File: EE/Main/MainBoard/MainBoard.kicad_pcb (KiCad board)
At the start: 2 copper layers, 135.8 x 87.5 mm, 59 parts, among them J1 Conn_01x04_Male, J2 Conn_01x04_Male, J3 Conn_01x04_Male, J4 Conn_01x04_Male, J5 Conn_01x04_Male, J6 Conn_01x04_Male, J7 TAG_CONNECT, J8 Conn_01x02_Male, P1 USB_C_Plug_USB2.0, Q1 2N7002NXAKR, Q2 2N7002NXAKR, Q3 2N7002NXAKR, Q4 2N7002NXAKR, SW1 EG1206A, U1 STM32C011F4U6TR, U2 DA04-11EWA, U3 DA04-11GWA, U4 MCP73832-2-OT, U5 TPS62172DSG

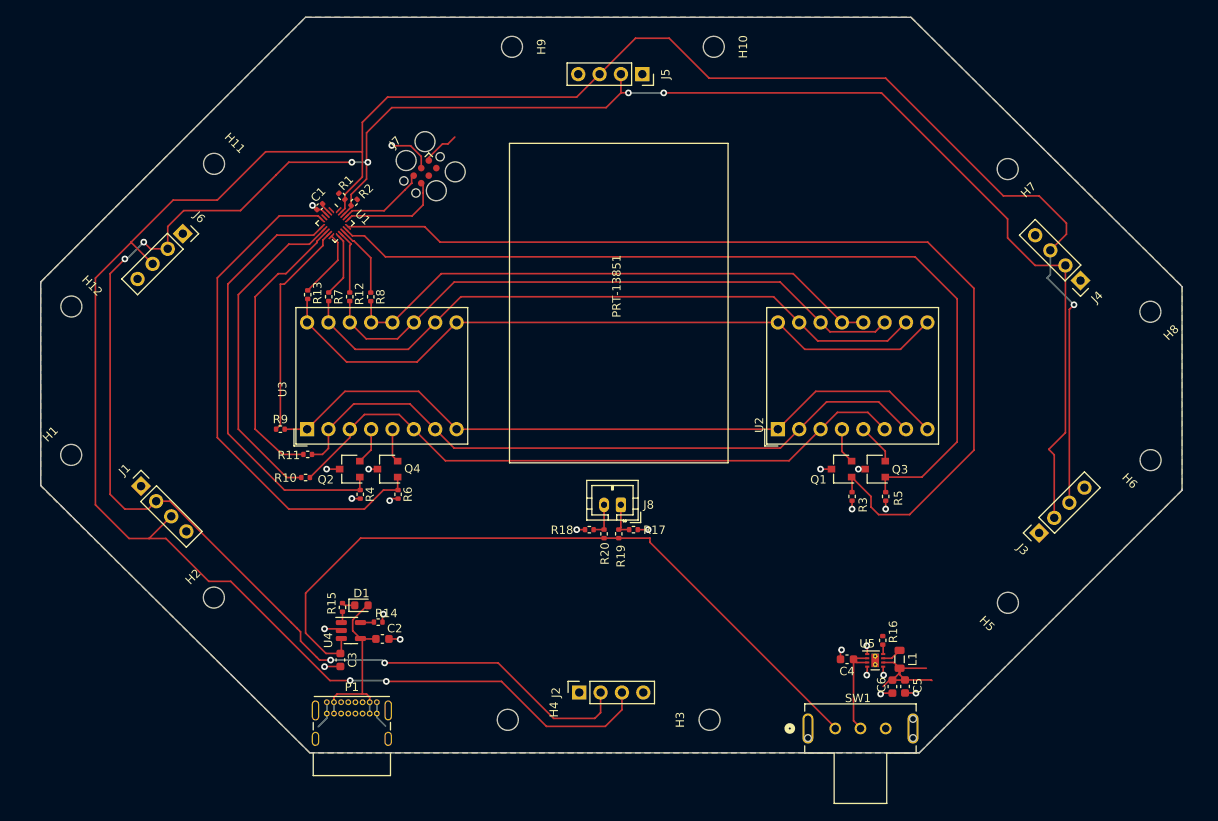
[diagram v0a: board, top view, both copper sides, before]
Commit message: Routine Update
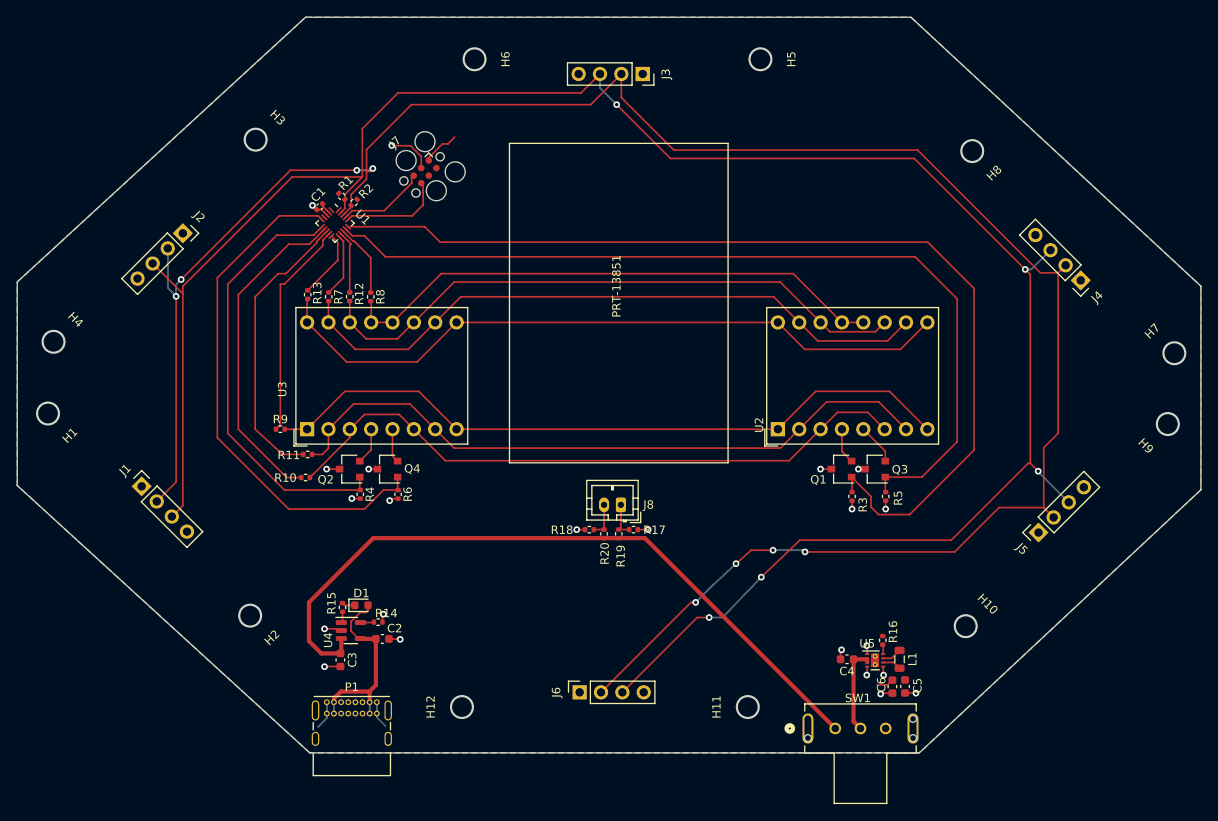
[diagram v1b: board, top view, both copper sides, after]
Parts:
- added ?: , , F.Cu at (159.6, 133.3)
- added ?: , , F.Cu at (186.3, 67.2)
- added ?: , , F.Cu at (77.0, 89.9)
- added ?: , , F.Cu at (76.4, 98.4)
- added ?: , , F.Cu at (100.4, 122.5)
- added ?: , , F.Cu at (210.3, 91.2)
- added ?: , , F.Cu at (127.1, 56.3)
- added ?: , , F.Cu at (185.5, 123.7)
- added ?: , , F.Cu at (161.1, 56.3)
- added ?: , , F.Cu at (125.6, 133.3)
- added ?: , , F.Cu at (209.6, 99.7)
- added ?: , , F.Cu at (101.1, 65.8)
- H1, H10, H11, H12, H2, H3, H4, H5, H6, H7, H8, H9: footprint MountingHole:MountingHole_2.5mm -> MountingHole:MountingHole_2.7mm
- moved H6 93.5 mm to (127.1, 56.3), turned to -90 degrees
- moved H11 90.6 mm to (159.6, 133.3), turned to 90 degrees
- moved H9 90.0 mm to (209.6, 99.7), turned to 135 degrees
- moved H3 87.6 mm to (101.1, 65.8), turned to -45 degrees
- moved H10 75.1 mm to (185.5, 123.7), turned to -45 degrees
- moved J2 72.2 mm to (92.4, 77.0), turned to -45 degrees
- moved J6 72.1 mm to (139.6, 131.6), turned to 90 degrees
- moved J3 72.1 mm to (147.1, 58.0), turned to -90 degrees
- moved J5 72.1 mm to (194.2, 112.6), turned to 135 degrees
- moved H5 71.0 mm to (161.1, 56.3), turned to -90 degrees
- moved H4 70.3 mm to (77.0, 89.9), turned to -45 degrees
- moved H12 66.5 mm to (125.6, 133.3), turned to 90 degrees
- moved H7 29.5 mm to (210.3, 91.2), turned to 45 degrees
- moved H8 28.5 mm to (186.3, 67.2)
- moved H1 5.64 mm to (76.4, 98.4), turned to -135 degrees
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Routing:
- net /SDA: track 293.3 -> 256.6 mm, vias 3 -> 5
- net /SCL: track 277.4 -> 262.6 mm
- net VCC: track 20.8 -> 10.4 mm
- net VBUS: track 22.2 -> 24.2 mm
- net /Power/V_PRE_REG: track 11.9 -> 10.7 mm
- net /Power/VBAT: track 87.1 -> 85.9 mm
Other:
- board size 135.8 x 87.5 mm -> 140.8 x 87.5 mm

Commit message: Random Check in
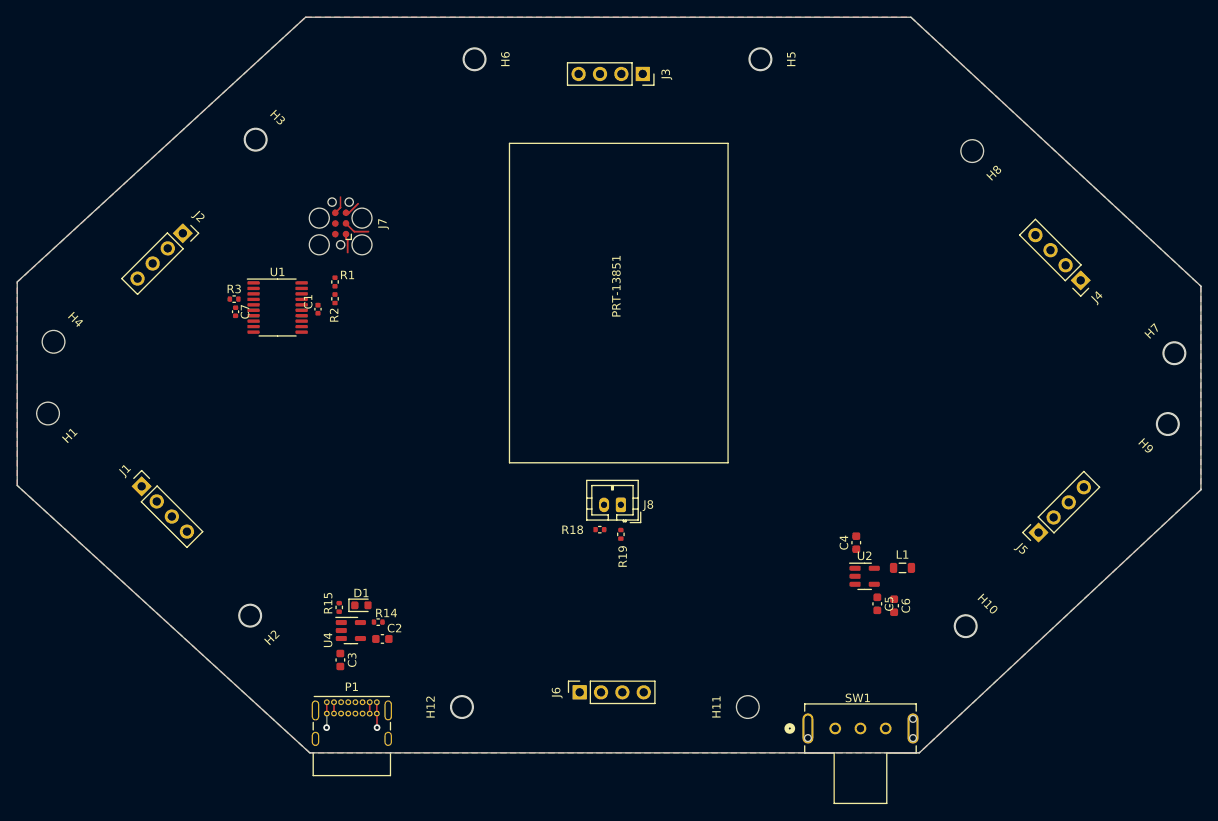
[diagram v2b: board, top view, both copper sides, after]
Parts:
- removed the ? at (159.6, 133.3)
- removed the ? at (186.3, 67.2)
- removed the ? at (77.0, 89.9)
- removed the ? at (76.4, 98.4)
- removed Q1, Q2, Q3, Q4: 2N7002NXAKR, Package_TO_SOT_SMD:SC-59
- removed R10, R11, R12, R13, R7, R8, R9: 560, Resistor_SMD:R_0402_1005Metric
- removed R16: 100k, Resistor_SMD:R_0402_1005Metric
- removed R17, R20: 0, Resistor_SMD:R_0402_1005Metric
- removed R4, R5, R6: 10k, Resistor_SMD:R_0402_1005Metric
- removed U3: DA04-11GWA, Display_7Segment:DA04-11CGKWA
- removed U5: TPS62172DSG, Package_SON:WSON-8-1EP_2x2mm_P0.5mm_EP0.9x1.6mm_ThermalVias
- added C7: 0.1u, Capacitor_SMD:C_0402_1005Metric, F.Cu at (98.7, 86.3)
- L1: value 2.2u -> 10u
- R14: value 20k -> 10k
- U1: value STM32C011F4U6TR -> STM32F030F4Px; footprint Package_DFN_QFN:UQFN-20_3x3mm_P0.4mm -> Package_SO:TSSOP-20_4.4x6.5mm_P0.65mm
- U2: value DA04-11EWA -> LM3670MF-3.3; footprint Display_7Segment:DA04-11SURKWA -> Package_TO_SOT_SMD:TSOT-23-5
- moved R3 77.2 mm to (98.5, 84.8), turned to 0 degrees
- moved U2 20.3 mm to (173.5, 117.8), turned to 0 degrees
- moved C4 13.9 mm to (172.5, 113.8), turned to 90 degrees
- moved C1 12.2 mm to (108.5, 86.0), turned to -90 degrees
- moved U1 12.1 mm to (103.7, 85.8), turned to 0 degrees
- moved J7 11.8 mm to (111.2, 75.8), turned to 90 degrees
- moved R2 11.7 mm to (110.5, 84.8), turned to 90 degrees
- moved L1 10.9 mm to (178.0, 116.8), turned to 0 degrees
- moved C5 10.4 mm to (175.0, 121.1)
- moved R1 10.2 mm to (110.5, 82.8), turned to -90 degrees
- moved C6 9.62 mm to (177.0, 121.3)
- moved R18 1.25 mm to (142.0, 112.2)
- moved R15 0.39 mm to (111.0, 121.5)
- moved R19 0.26 mm to (144.5, 112.8)
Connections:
- C4 pad 1: /Power/V_PRE_REG -> /Power/V_DISPLAY
- R3 pad 1: /Display/D1_R_EN -> VCC
- R3 pad 2: GND -> Net-(R3-Pad2)
- SW1 pad 2: /Power/V_PRE_REG -> /Power/V_DISPLAY
- U1 pad 10: /Display/G_EN -> unconnected-(U1-Pad10)
- U1 pad 11: /Display/A_EN -> /MCU/DNC_SPI_CLK
- U1 pad 12: /Display/F_EN -> unconnected-(U1-Pad12)
- U1 pad 13: /Display/B_EN -> /Display/DISPLAY_DIN
- U1 pad 14: /Display/D2_R_EN -> unconnected-(U1-Pad14)
- U1 pad 15: /Display/D1_R_EN -> GND
- U1 pad 16: /MCU/SWDIO -> VCC
- U1 pad 17: /MCU/SWDCLK -> /SCL
- U1 pad 18: /SCL -> /SDA
- U1 pad 19: /SDA -> /MCU/SWDIO
- U1 pad 2: VCC -> unconnected-(U1-Pad2)
- U1 pad 20: unconnected-(U1-Pad20) -> /MCU/SWDCLK
- U1 pad 3: GND -> unconnected-(U1-Pad3)
- U1 pad 4: unconnected-(U1-Pad4) -> Net-(R3-Pad2)
- U1 pad 5: /Display/D2_G_EN -> VCC
- U1 pad 6: /Display/D1_G_EN -> unconnected-(U1-Pad6)
- U1 pad 7: /Display/D_EN -> unconnected-(U1-Pad7)
- U1 pad 8: /Display/E_EN -> unconnected-(U1-Pad8)
- U1 pad 9: /Display/C_EN -> unconnected-(U1-Pad9)
- U2 pad 1: /Display/C -> /Power/V_DISPLAY
- U2 pad 2: /Display/E -> GND
- U2 pad 3: /Display/D -> /Power/V_DISPLAY
- U2 pad 4: /Display/D1_R -> VCC
- U2 pad 5: /Display/D2_R -> Net-(L1-Pad1)
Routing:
- net /SCL: track 262.6 -> 0.00 mm, vias 8 -> 0
- net /SDA: track 256.6 -> 0.00 mm, vias 5 -> 0
- net /Display/D1_R_EN: track 118.9 -> 0.00 mm
- net /Display/D2_R_EN: track 105.3 -> 0.00 mm
- net /Power/VBAT: track 85.9 -> 0.00 mm
- net /Display/C: track 83.9 -> 0.00 mm
- net /Display/G: track 83.1 -> 0.00 mm
- net /Display/E: track 80.3 -> 0.00 mm
- net /Display/A: track 78.3 -> 0.00 mm
- net /Display/D: track 77.5 -> 0.00 mm
- net /Display/F: track 72.7 -> 0.00 mm
- net /Display/B: track 65.9 -> 0.00 mm
- net /Display/D2_G_EN: track 62.2 -> 0.00 mm
- net /Display/D1_G_EN: track 51.9 -> 0.00 mm
- net /Display/D_EN: track 39.3 -> 0.00 mm
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- added copper zone on F.Cu, net GND
- removed copper zone on F.Cu, net VCC
